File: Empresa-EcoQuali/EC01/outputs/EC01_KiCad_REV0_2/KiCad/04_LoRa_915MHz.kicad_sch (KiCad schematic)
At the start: 10 parts, among them J1 U.FL-R-SMT-1, U3 E22-900M22S SX1262

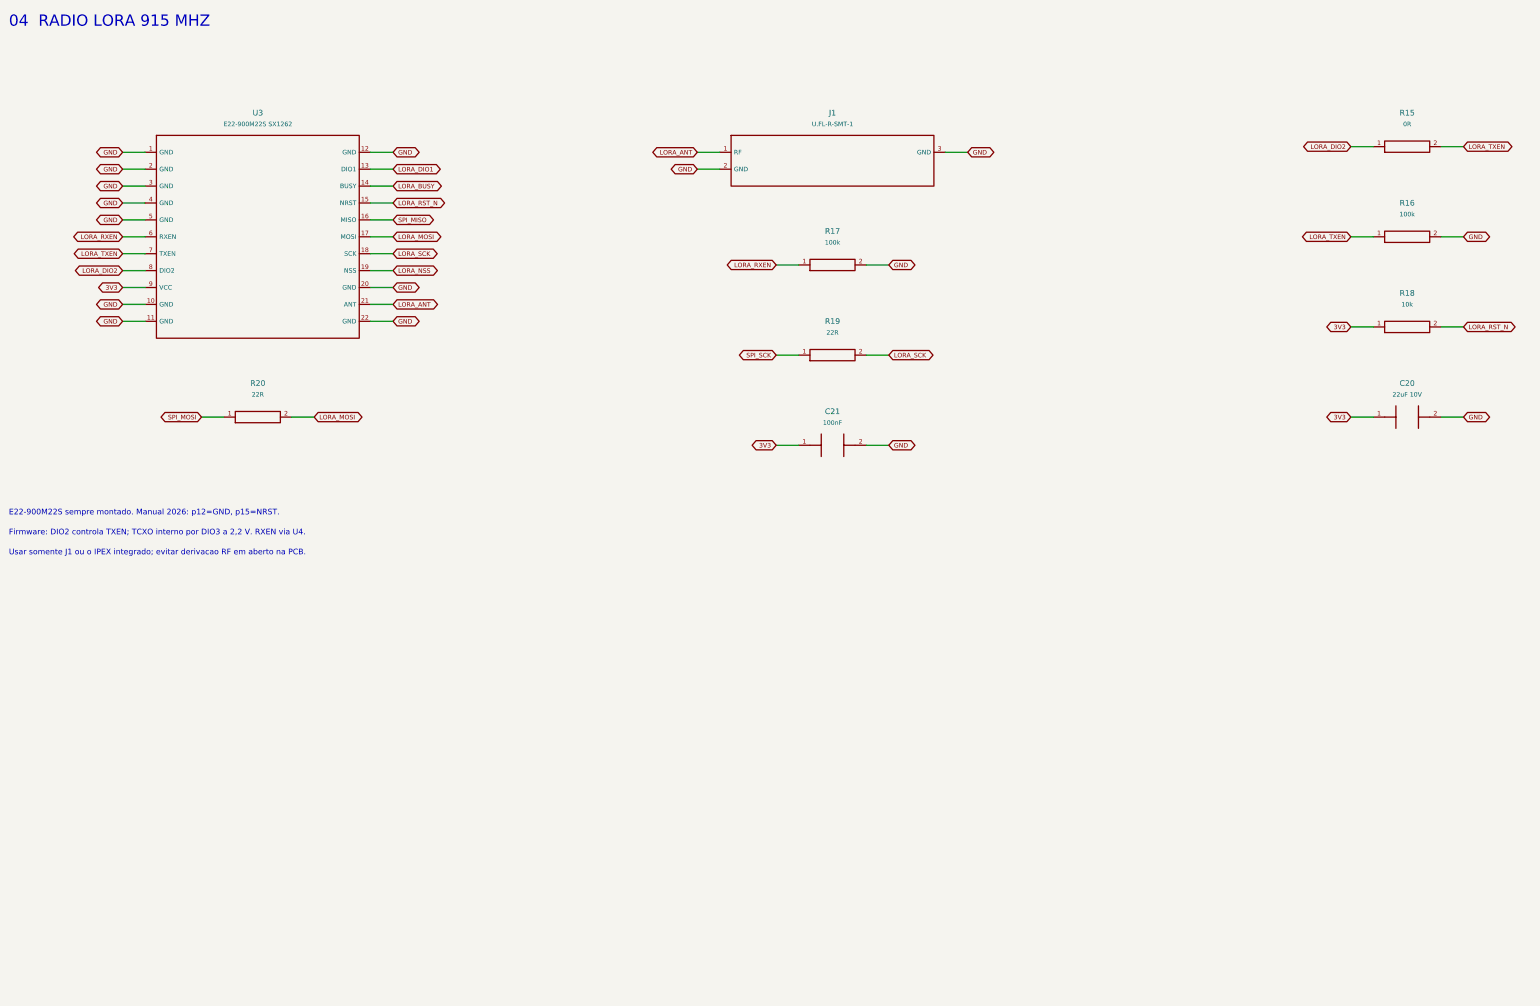
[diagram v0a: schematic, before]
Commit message: EC01
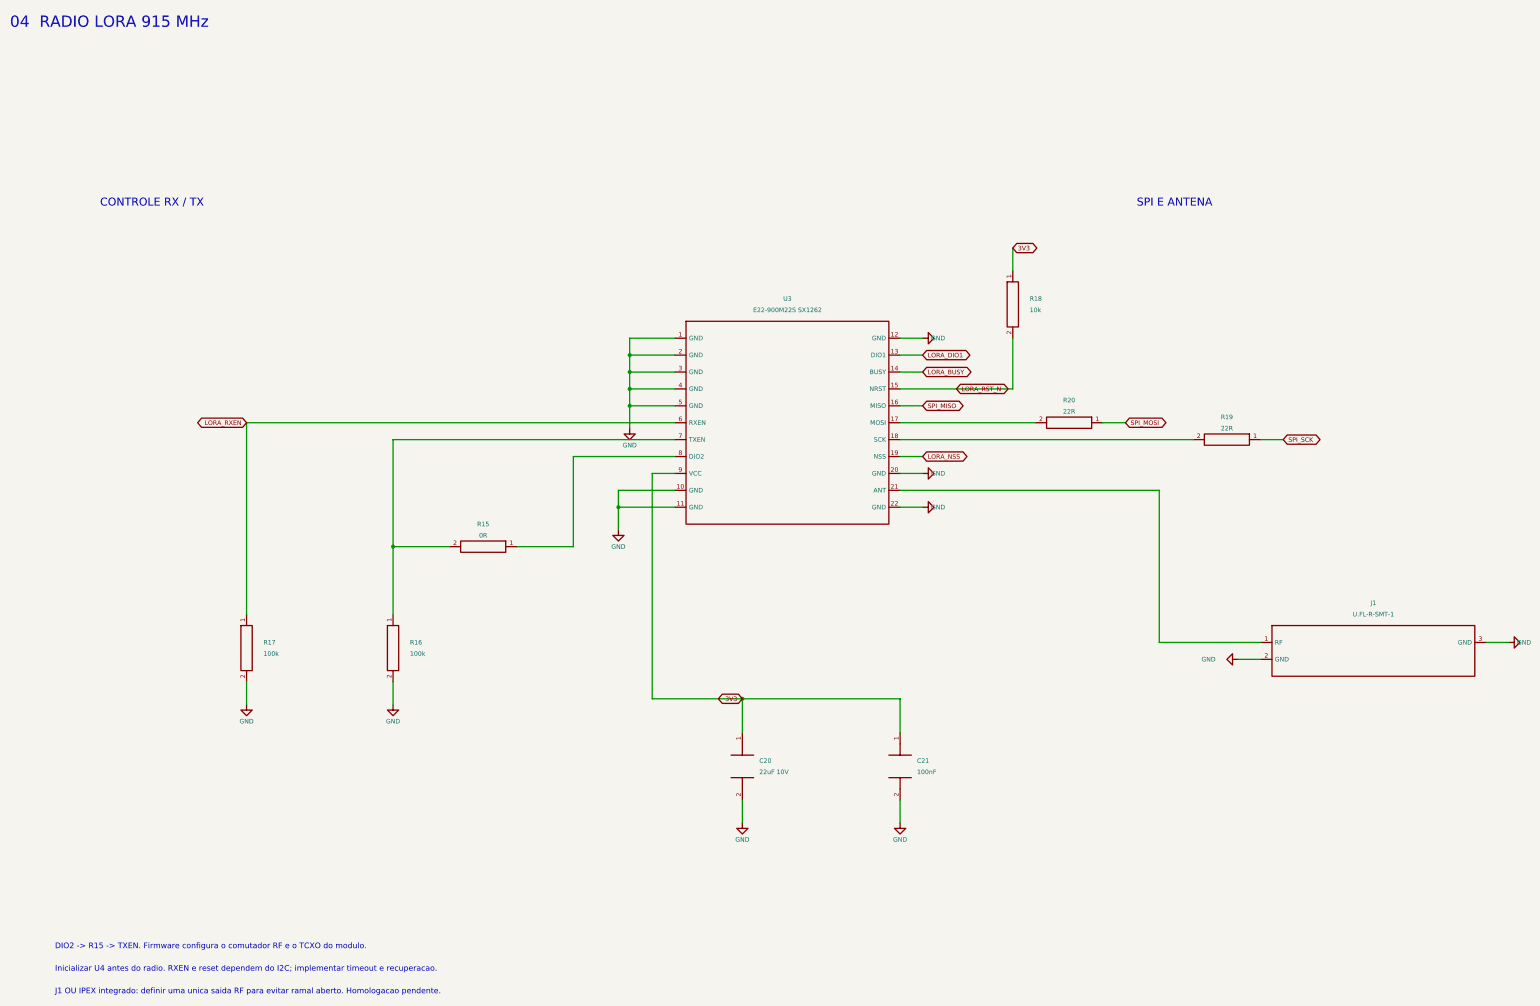
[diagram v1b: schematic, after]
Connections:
- net LORA_ANT: no longer names the net of J1.1 (RF), U3.21 (ANT)
- net LORA_DIO2: no longer names the net of R15.1, U3.8 (DIO2)
- net LORA_MOSI: no longer names the net of R20.2, U3.17 (MOSI)
- net LORA_SCK: no longer names the net of R19.2, U3.18 (SCK)
- net LORA_TXEN: no longer names the net of R15.2, R16.1, U3.7 (TXEN)
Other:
- note added: "04 RADIO LORA 915 MHz"
- note added: "CONTROLE RX / TX"
- note added: "DIO2 -> R15 -> TXEN. Firmware configura o comutador RF e o TCXO do modulo."
- note added: "Inicializar U4 antes do radio. RXEN e reset dependem do I2C; implementar timeout e recuperacao."
- note added: "J1 OU IPEX integrado: definir uma unica saida RF para evitar ramal aberto. Homologacao pendente."
- note added: "SPI E ANTENA"
- note removed: "04 RADIO LORA 915 MHZ"
- note removed: "E22-900M22S sempre montado. Manual 2026: p12=GND, p15=NRST."
- note removed: "Firmware: DIO2 controla TXEN; TCXO interno por DIO3 a 2,2 V. RXEN via U4."
- note removed: "Usar somente J1 ou o IPEX integrado; evitar derivacao RF em aberto na PCB."
- moved on the sheet: C20, C21, J1, R15, R16, R17, R18, R19, R20, U3
